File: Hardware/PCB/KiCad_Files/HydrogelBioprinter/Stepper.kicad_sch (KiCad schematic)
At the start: 31 parts, among them J17 Conn_01x04_Pin, J18 Conn_01x04_Pin, J19 Conn_01x04_Pin, J20 Conn_01x04_Pin, J21 Conn_01x04_Pin

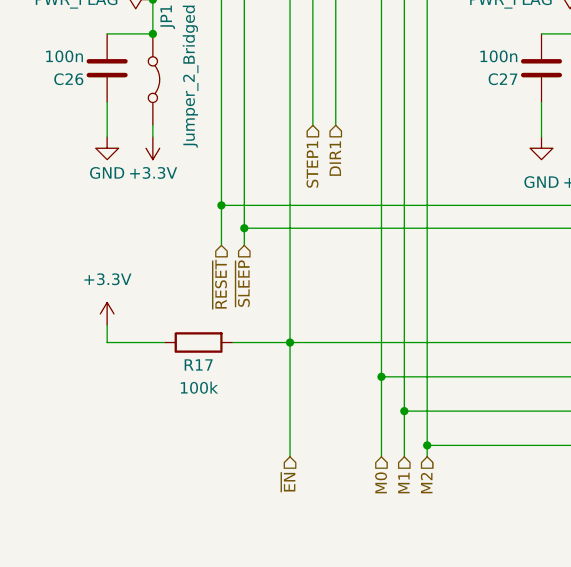
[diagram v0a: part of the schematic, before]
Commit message: Gantry Concept 1 Completion and PCB schematic update
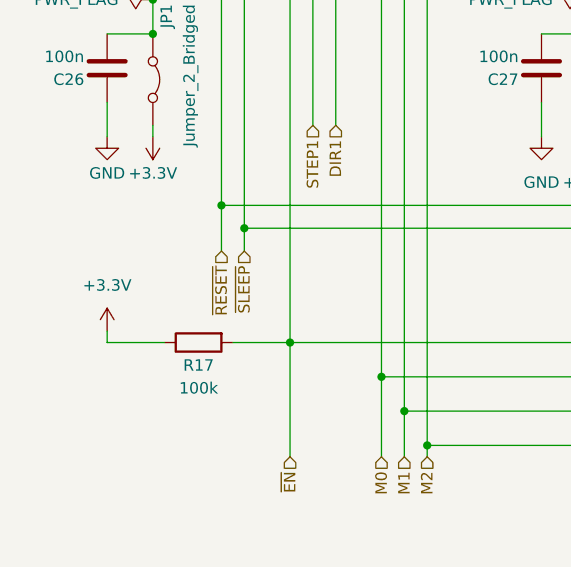
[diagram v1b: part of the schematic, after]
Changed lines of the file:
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@@
 	(wire
 		(pts
-			(xy 33.02 112.395) (xy 33.02 114.3)
+			(xy 33.02 113.03) (xy 33.02 114.3)
 		)
 		(stroke
@@
 	(wire
 		(pts
-			(xy 48.26 101.6) (xy 48.26 103.505)
+			(xy 48.26 101.6) (xy 48.26 104.14)
 		)
 		(stroke
@@
 	(wire
 		(pts
-			(xy 45.72 99.06) (xy 45.72 103.505)
+			(xy 45.72 99.06) (xy 45.72 104.14)
 		)
 		(stroke
@@
 	(hierarchical_label "~{SLEEP}"
 		(shape input)
-		(at 48.26 103.505 270)
+		(at 48.26 104.14 270)
 		(effects
 			(font
@@
 	(hierarchical_label "~{RESET}"
 		(shape input)
-		(at 45.72 103.505 270)
+		(at 45.72 104.14 270)
 		(effects
 			(font
@@
 	(symbol
 		(lib_id "power:+3.3V")
-		(at 33.02 112.395 0)
+		(at 33.02 113.03 0)
 		(mirror y)
 		(unit 1)
@@
 		(fields_autoplaced yes)
 		(property "Reference" "#PWR069"
-			(at 33.02 116.205 0)
+			(at 33.02 116.84 0)
 			(effects
 				(font
@@
 		)
 		(property "Value" "+3.3V"
-			(at 33.02 107.315 0)
+			(at 33.02 107.95 0)
 			(effects
 				(font
@@
 		)
 		(property "Footprint" ""
-			(at 33.02 112.395 0)
+			(at 33.02 113.03 0)
 			(effects
 				(font
@@
 		)
 		(property "Datasheet" ""
-			(at 33.02 112.395 0)
+			(at 33.02 113.03 0)
 			(effects
 				(font
@@
 		)
 		(property "Description" "Power symbol creates a global label with name \"+3.3V\""
-			(at 33.02 112.395 0)
-			(effects
-				(font
+			(at 33.02 113.03 0)
+			(effects
+				(font
